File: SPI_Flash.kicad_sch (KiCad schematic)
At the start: 1 part, among them U1 W25Q32JVSS

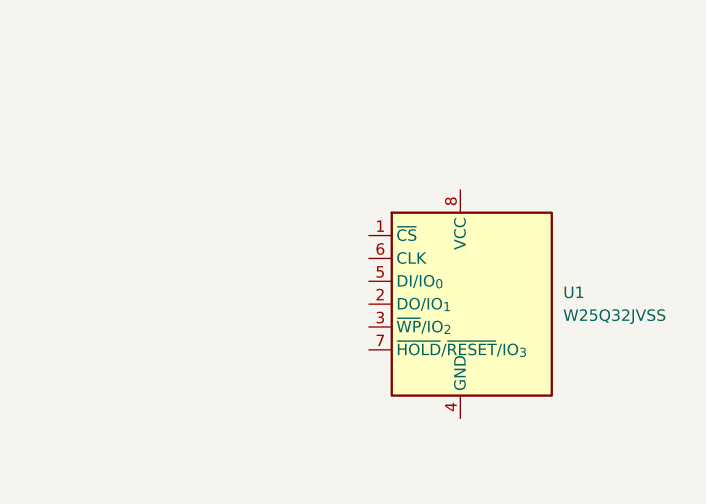
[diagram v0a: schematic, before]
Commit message: init_sch
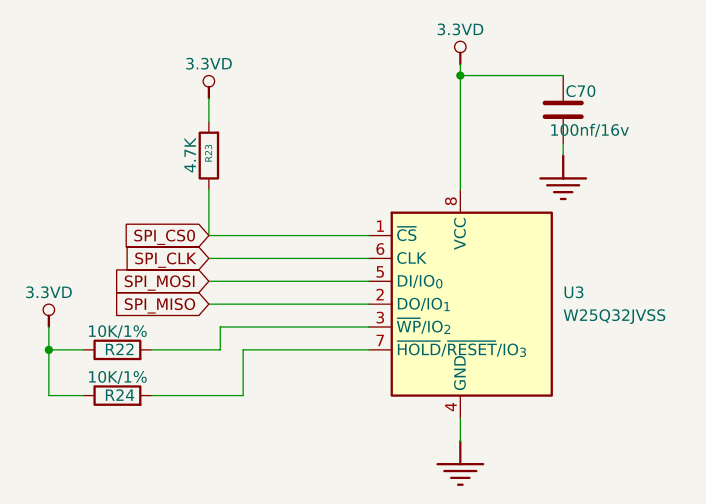
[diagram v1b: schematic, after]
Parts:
- added C70: 100nf/16v, symbol Device:C
- added R22, R24: 10K/1%, symbol Device:R
- added R23: 4.7K, Resistor_SMD:R_0402_1005Metric, symbol Device:R
- renumbered U1 to U3
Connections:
- net SPI_CS0: now reaches U3.1 (~{CS})
- net SPI_CS0: now also R23.1
- net SPI_MISO: now reaches U3.2 (DO/IO_{1})
- net at U3.3 (~{WP}/IO_{2}): now also R22.2
- net GND: now reaches U3.4 (GND)
- net GND: now also C70.2
- net SPI_MOSI: now reaches U3.5 (DI/IO_{0})
- net SPI_CLK: now reaches U3.6 (CLK)
- net at U3.7 (~{HOLD}/~{RESET}/IO_{3}): now also R24.2
- net 3.3VD: now reaches U3.8 (VCC)
- net 3.3VD: now also C70.1, R22.1, R23.2, R24.1

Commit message: updated
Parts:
- C70: footprint (none) -> Capacitor_SMD:C_0402_1005Metric; LCSC (none) -> C1525
- R22, R24: footprint (none) -> Resistor_SMD:R_0402_1005Metric; LCSC (none) -> C25744
- U3: footprint Package_SO:SOIC-8_5.3x5.3mm_P1.27mm -> Package_SO:SOIC-8-1EP_3.9x4.9mm_P1.27mm_EP2.29x3mm_ThermalVias; LCSC (none) -> C82344
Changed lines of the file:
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@@
 			)
 		)
-		(property "Footprint" ""
+		(property "Footprint" "Resistor_SMD:R_0402_1005Metric"
 			(at 114.3 98.298 90)
 			(effects
@@
 			)
 		)
+		(property "LCSC" "C25744"
+			(at 114.3 96.52 90)
+			(effects
+				(font
+					(size 1.27 1.27)
+				)
+				(hide yes)
+			)
+		)
 		(pin "2"
 		)
@@
 			)
 		)
-		(property "Footprint" ""
+		(property "Footprint" "Capacitor_SMD:C_0402_1005Metric"
 			(at 164.7952 73.66 0)
 			(effects
@@
 			)
 		)
+		(property "LCSC" "C1525"
+			(at 163.83 69.85 0)
+			(effects
+				(font
+					(size 1.27 1.27)
+				)
+				(hide yes)
+			)
+		)
 		(pin "2"
 		)
@@
 			)
 		)
-		(property "Footprint" ""
+		(property "Footprint" "Resistor_SMD:R_0402_1005Metric"
 			(at 114.3 103.378 90)
 			(effects
@@
 		(property "Description" "Resistor"
 			(at 114.3 101.6 0)
+			(effects
+				(font
+					(size 1.27 1.27)
+				)
+				(hide yes)
+			)
+		)
+		(property "LCSC" "C25744"
+			(at 114.3 101.6 90)
 			(effects
 				(font
@@
 			)
 		)
-		(property "Footprint" "Package_SO:SOIC-8_5.3x5.3mm_P1.27mm"
+		(property "Footprint" "Package_SO:SOIC-8-1EP_3.9x4.9mm_P1.27mm_EP2.29x3mm_ThermalVias"
 			(at 152.4 91.44 0)
 			(effects
@@
 			(at 152.4 91.44 0)
 			(effects
+				(font
+					(size 1.27 1.27)
+				)
+				(hide yes)
+			)
+		)
+		(property "LCSC" "C82344"
+			(at 152.4 91.44 0)
+			(effects
